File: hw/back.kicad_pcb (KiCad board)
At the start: 2 copper layers, 110 x 55 mm, 77 parts, among them J1 IDC_02X13, J2 FC681495, J3 N42GK-04, Q1 BSC080N03MS, U1 OSRB38C9BA, U2 MCP1826S, U3 MCP1826S, U4 BQ24192, U5 LTC1871, U6 LTC2941CMS8E

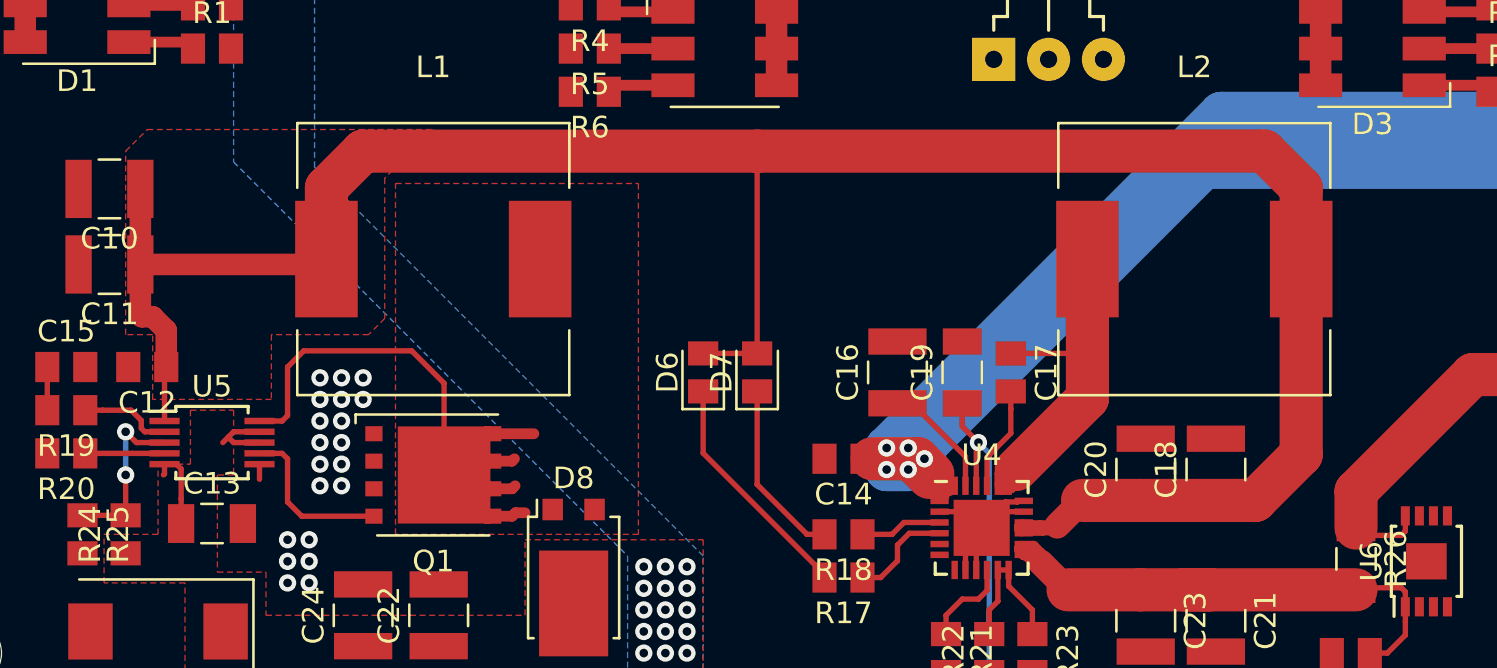
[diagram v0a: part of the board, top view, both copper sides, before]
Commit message: updated pcb
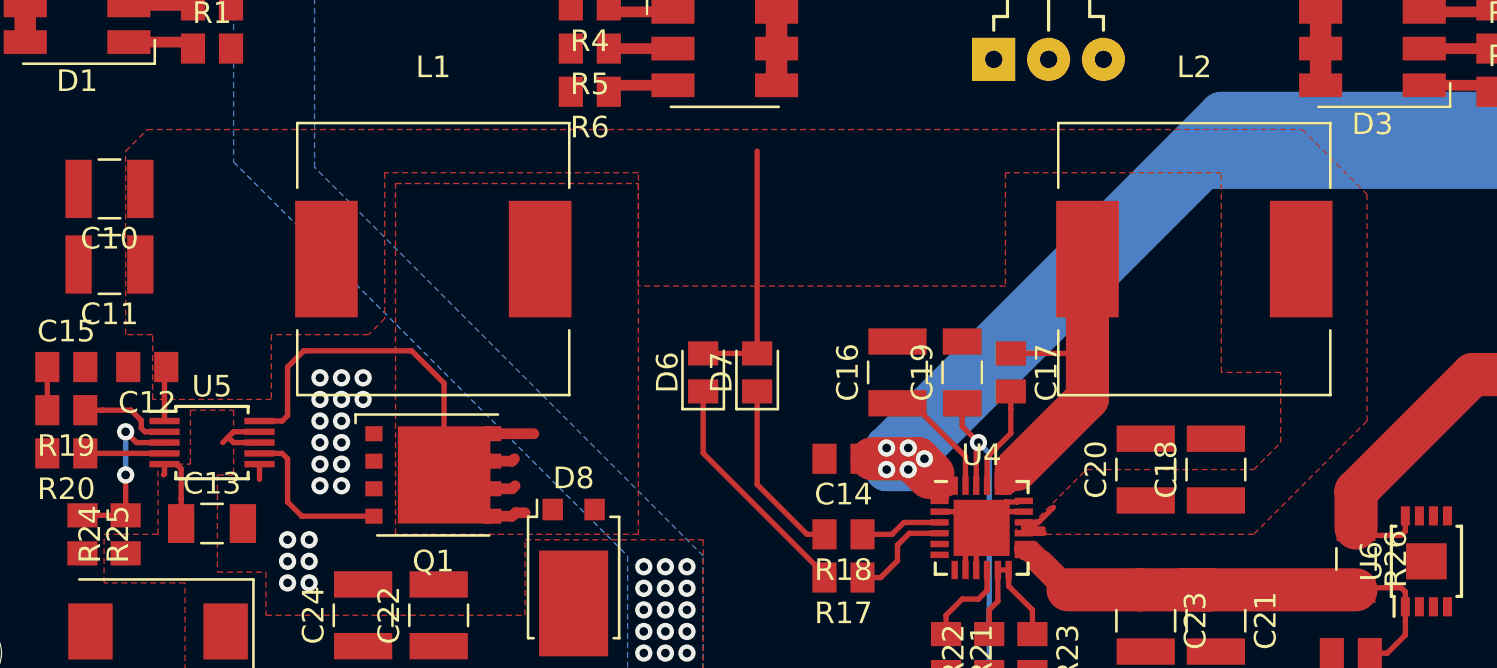
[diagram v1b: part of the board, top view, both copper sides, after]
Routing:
- net +BATT: track 118.2 -> 20.3 mm
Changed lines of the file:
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@@
     (thickness 1.6)
     (drawings 6)
-    (tracks 406)
+    (tracks 381)
     (zones 0)
     (modules 77)
@@
     (mod_text_size 1 1)
     (mod_text_width 0.15)
-    (pad_size 1.22 2.7)
+    (pad_size 0.85 0.3)
     (pad_drill 0)
     (pad_to_mask_clearance 0.2)
@@
       (net 2 /charger/BAT))
     (pad 15 smd rect (at 1.95 0.25) (size 0.85 0.3) (layers F.Cu F.Paste F.Mask)
-      (net 31 +BATT))
+      (net 31 +BATT) (zone_connect 2))
     (pad 16 smd rect (at 1.95 -0.25) (size 0.85 0.3) (layers F.Cu F.Paste F.Mask)
-      (net 31 +BATT))
+      (net 31 +BATT) (zone_connect 2))
     (pad 17 smd rect (at 1.95 -0.75) (size 0.85 0.3) (layers F.Cu F.Paste F.Mask)
       (net 5 GND))
@@
   (segment (start 132.5 94.36) (end 131.94 93.8) (width 0.5) (layer F.Cu) (net 29))
   (segment (start 132.5 96.37) (end 132.5 94.36) (width 0.5) (layer F.Cu) (net 29))
-  (segment (start 102.93 117) (end 111.3 117) (width 1) (layer F.Cu) (net 31))
+  (segment (start 143.85 129.45) (end 143.85 128.95) (width 0.25) (layer F.Cu) (net 31))
+  (segment (start 144.4 129) (end 144.1 129) (width 0.25) (layer F.Cu) (net 31))
+  (segment (start 144.1 129) (end 143.85 129.25) (width 0.25) (layer F.Cu) (net 31))
+  (segment (start 144.45 128.95) (end 144.4 129) (width 0.25) (layer F.Cu) (net 31))
+  (segment (start 143.85 128.95) (end 144.45 128.95) (width 0.25) (layer F.Cu) (net 31))
+  (segment (start 143.85 129.25) (end 144.75 129.25) (width 0.25) (layer F.Cu) (net 31))
+  (segment (start 143.85 129.45) (end 143.85 129.25) (width 0.25) (layer F.Cu) (net 31))
+  (segment (start 143.85 129.45) (end 144.8 129.45) (width 0.25) (layer F.Cu) (net 31))
+  (segment (start 143.85 128.95) (end 144.525 128.95) (width 0.25) (layer F.Cu) (net 31))
+  (segment (start 144.525 128.95) (end 145.225 128.25) (width 0.25) (layer F.Cu) (net 31))
   (segment (start 111.3 117) (end 111.55 116.75) (width 1) (layer F.Cu) (net 31))
-  (segment (start 102.93 113.5) (end 102.93 117) (width 1) (layer F.Cu) (net 31))
-  (segment (start 103.5 119.42) (end 103 119.42) (width 1) (layer F.Cu) (net 31))
-  (segment (start 103 119.42) (end 102.93 119.35) (width 1) (layer F.Cu) (net 31))
-  (segment (start 102.93 119.35) (end 102.93 117) (width 1) (layer F.Cu) (net 31))
-  (segment (start 104.13 121.75) (end 104.13 120.05) (width 1) (layer F.Cu) (net 31))
-  (segment (start 104.13 120.05) (end 103.5 119.42) (width 1) (layer F.Cu) (net 31))
   (segment (start 104.05 124.25) (end 104.05 121.83) (width 0.25) (layer F.Cu) (net 31))
   (segment (start 104.05 121.83) (end 104.13 121.75) (width 0.25) (layer F.Cu) (net 31))
   (segment (start 129 121.12) (end 129.95 121.12) (width 0.25) (layer F.Cu) (net 31))
   (segment (start 129.95 121.12) (end 131.5 121.12) (width 0.25) (layer F.Cu) (net 31))
-  (segment (start 113.25 111.75) (end 131.5 111.75) (width 2) (layer F.Cu) (net 31))
-  (segment (start 131.5 111.75) (end 155 111.75) (width 2) (layer F.Cu) (net 31))
   (segment (start 131.5 121.12) (end 131.5 111.75) (width 0.25) (layer F.Cu) (net 31))
-  (segment (start 152.75 127.93) (end 148 127.93) (width 0.5) (layer F.Cu) (net 31))
-  (segment (start 148 127.93) (end 149.5 127.93) (width 0.5) (layer F.Cu) (net 31))
-  (segment (start 156.7 116.75) (end 156.7 125.8) (width 2) (layer F.Cu) (net 31))
-  (segment (start 156.7 125.8) (end 154.57 127.93) (width 2) (layer F.Cu) (net 31))
-  (segment (start 154.57 127.93) (end 149.25 127.93) (width 2) (layer F.Cu) (net 31))
-  (segment (start 149.25 127.93) (end 146.57 127.93) (width 2) (layer F.Cu) (net 31))
-  (segment (start 144.15 129.3) (end 145.2 129.3) (width 0.5) (layer F.Cu) (net 31))
-  (segment (start 145.2 129.3) (end 145.4 129.1) (width 0.5) (layer F.Cu) (net 31))
-  (segment (start 144.6 129.1) (end 144.6 129.15) (width 0.5) (layer F.Cu) (net 31))
-  (segment (start 144.6 129.15) (end 144.75 129.3) (width 0.5) (layer F.Cu) (net 31))
-  (segment (start 144.75 129.3) (end 144.15 129.3) (width 0.5) (layer F.Cu) (net 31))
-  (segment (start 144.6 129.1) (end 145.4 129.1) (width 0.5) (layer F.Cu) (net 31))
-  (segment (start 144.25 129.1) (end 144.6 129.1) (width 0.5) (layer F.Cu) (net 31))
-  (segment (start 144.15 129.2) (end 143.650001 129.2) (width 0.5) (layer F.Cu) (net 31))
-  (segment (start 144.15 129.2) (end 144.15 129.3) (width 0.5) (layer F.Cu) (net 31))
-  (segment (start 144.200001 129.149999) (end 144.25 129.1) (width 0.5) (layer F.Cu) (net 31))
-  (segment (start 143.650001 129.149999) (end 144.200001 129.149999) (width 0.5) (layer F.Cu) (net 31))
-  (segment (start 146.57 127.93) (end 145.4 129.1) (width 1.2) (layer F.Cu) (net 31))
-  (segment (start 143.650001 129.2) (end 143.650001 129.250001) (width 0.5) (layer F.Cu) (net 31))
-  (segment (start 143.650001 129.250001) (end 143.749999 129.349999) (width 0.5) (layer F.Cu) (net 31))
-  (segment (start 143.650001 129.2) (end 143.650001 129.149999) (width 0.5) (layer F.Cu) (net 31))
-  (segment (start 143.650001 129.149999) (end 143.749999 129.050001) (width 0.5) (layer F.Cu) (net 31))
-  (segment (start 155 111.75) (end 156.7 113.45) (width 2) (layer F.Cu) (net 31))
-  (segment (start 111.55 113.45) (end 113.25 111.75) (width 2) (layer F.Cu) (net 31))
-  (segment (start 111.55 116.75) (end 111.55 113.45) (width 2) (layer F.Cu) (net 31))
-  (segment (start 156.7 113.45) (end 156.7 116.75) (width 2) (layer F.Cu) (net 31))
   (segment (start 146.8 121.25) (end 146.8 123.2) (width 2) (layer F.Cu) (net 32))
   (segment (start 146.8 116.75) (end 146.8 121.25) (width 2) (layer F.Cu) (net 32))
@@
     (polygon
       (pts
-        (xy 102.25 111.75) (xy 103.25 110.75) (xy 116.5 110.75) (xy 114.25 113) (xy 114.25 119.5)
-        (xy 113.5 120.25) (xy 109 120.25) (xy 109 123.25) (xy 103.5 123.25) (xy 103.5 120.25)
-        (xy 102.25 120.25)
+        (xy 102.25 111.75) (xy 103.25 110.75) (xy 156.75 110.75) (xy 159.75 113.75) (xy 159.75 124.25)
+        (xy 154.5 129.5) (xy 144.25 129.5) (xy 143.5 129.5) (xy 143.5 129) (xy 144.25 129)
+        (xy 146.75 126.5) (xy 154.5 126.5) (xy 155.75 125.25) (xy 155.75 122) (xy 153 122)
+        (xy 153 112.75) (xy 143 112.75) (xy 143 118) (xy 126 118) (xy 126 112.75)
+        (xy 114.25 112.75) (xy 114.25 119.5) (xy 113.5 120.25) (xy 109 120.25) (xy 109 123.25)
+        (xy 103.5 123.25) (xy 103.5 120.25) (xy 102.25 120.25)
       )
     )
